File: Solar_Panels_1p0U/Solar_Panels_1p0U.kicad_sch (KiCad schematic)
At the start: 46 parts, among them J1 5040500891

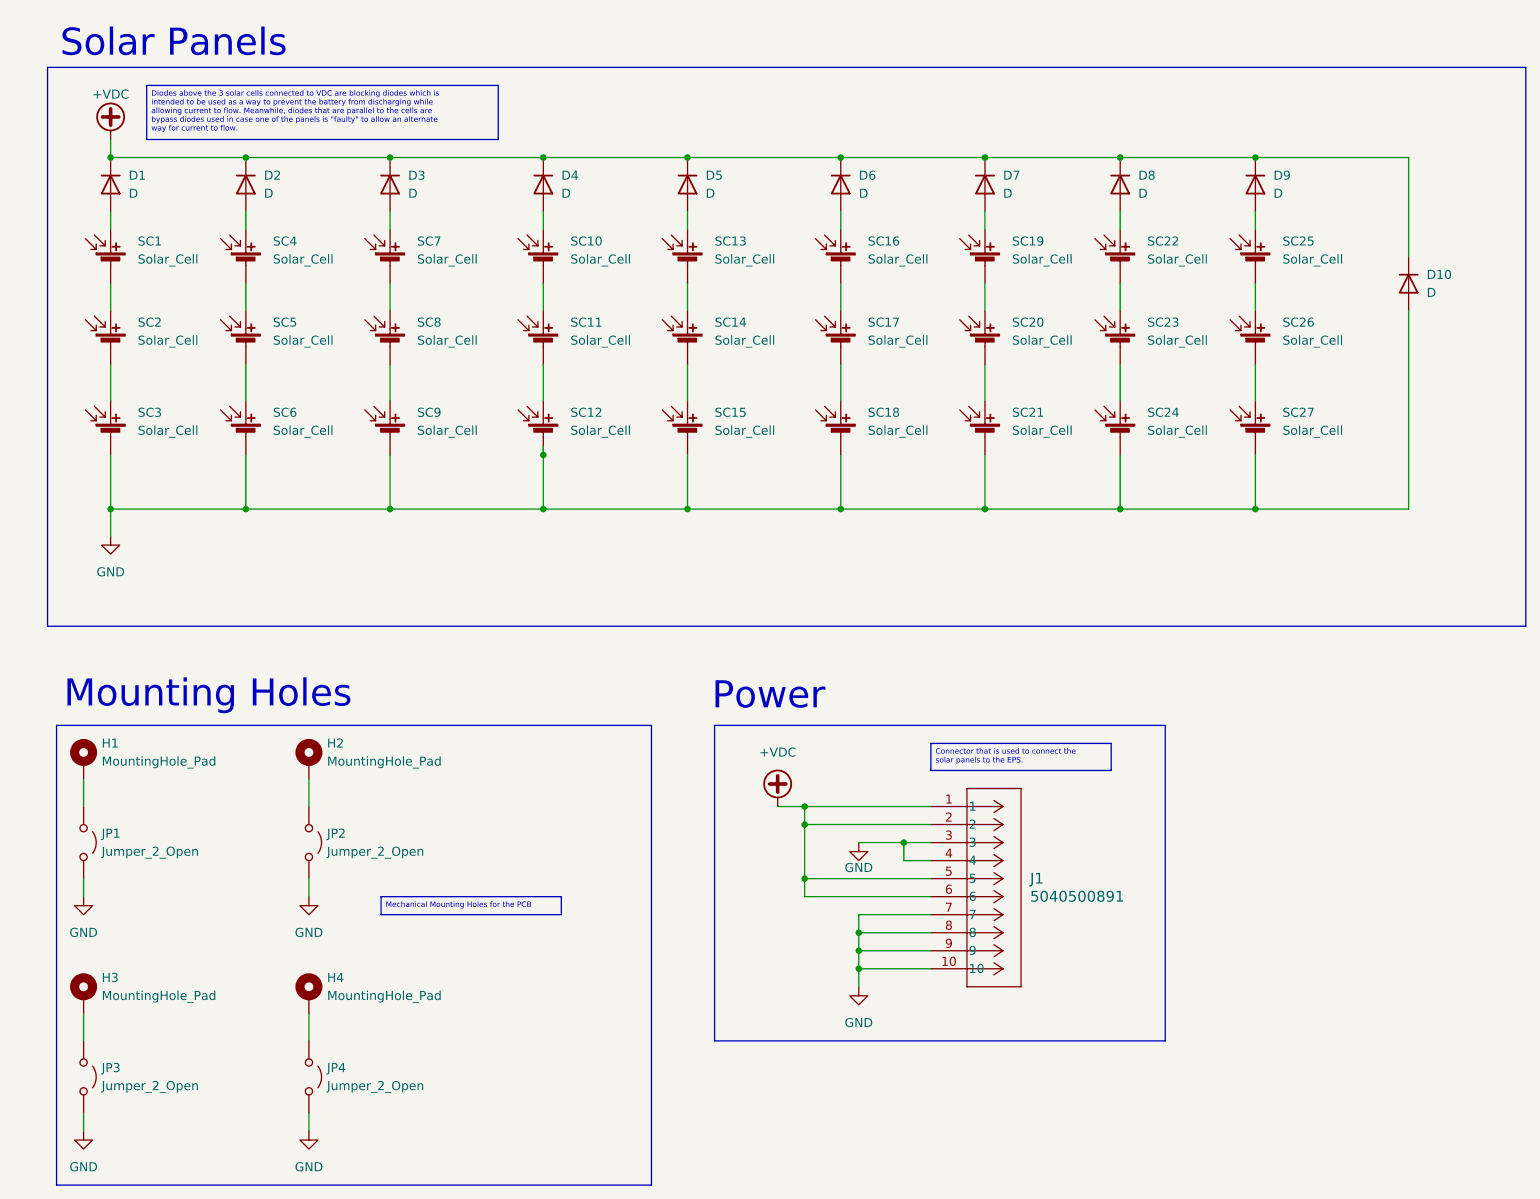
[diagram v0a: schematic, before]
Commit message: Kicad 9.0 PCB UPDATE
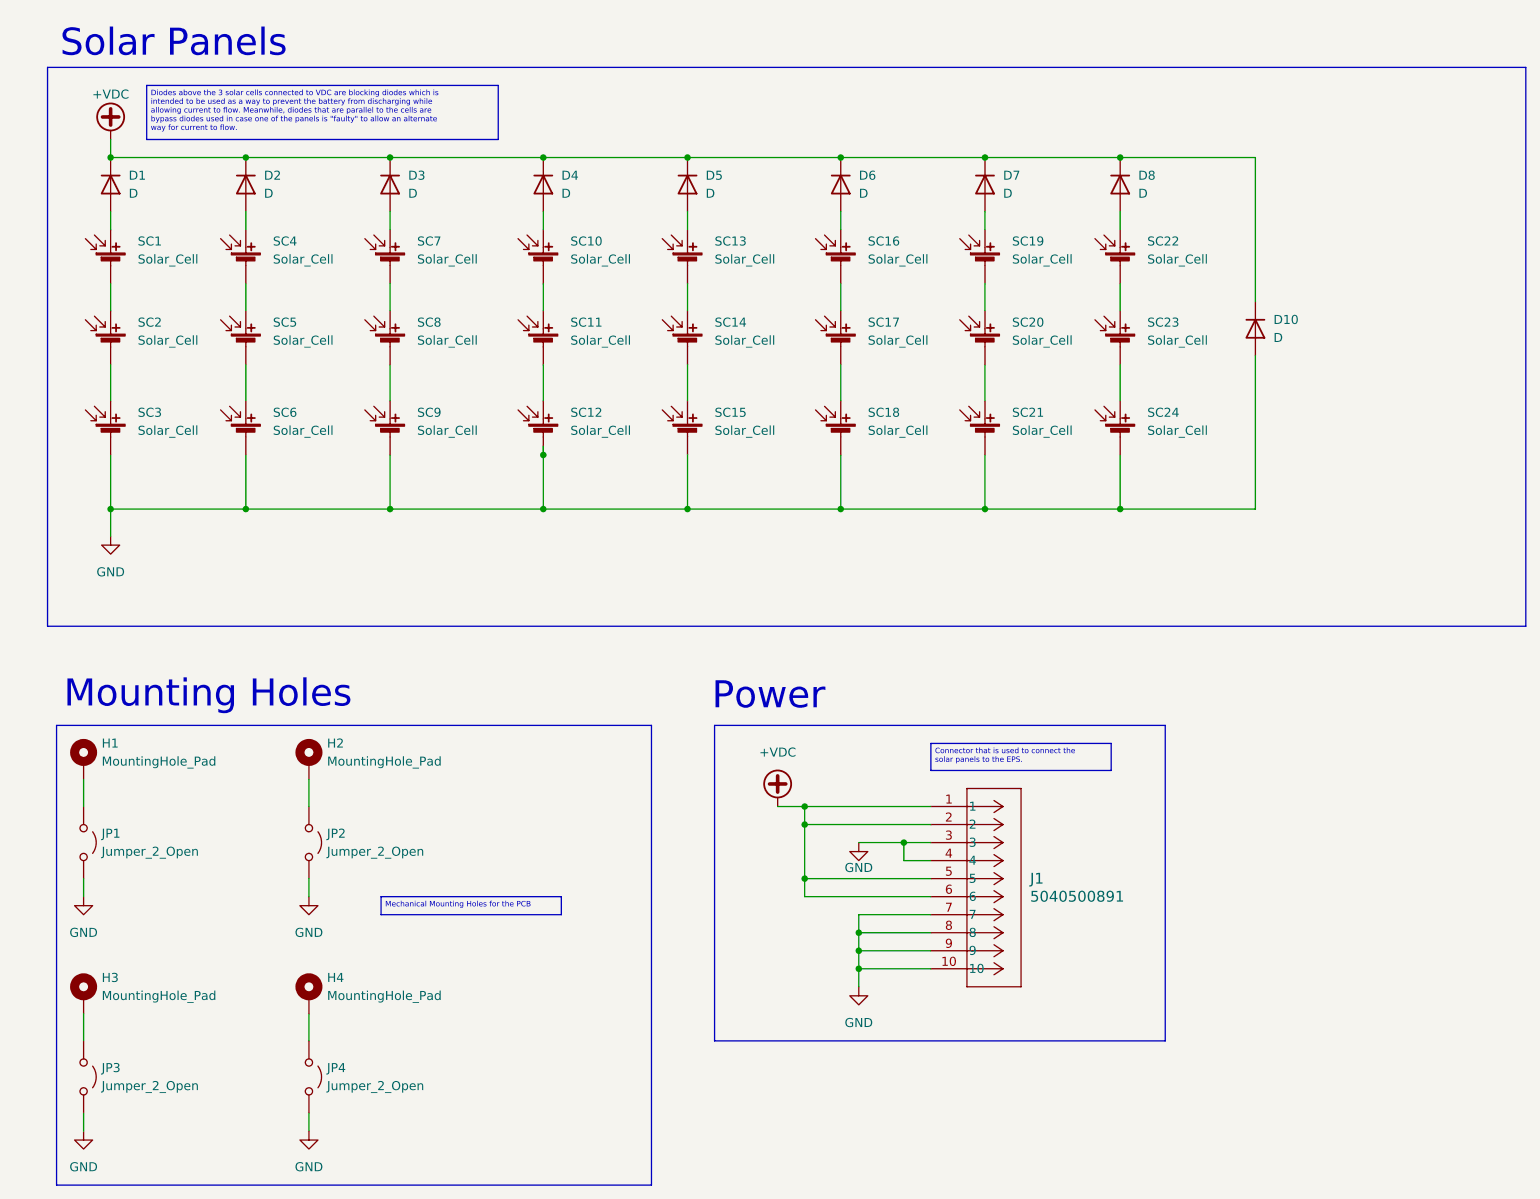
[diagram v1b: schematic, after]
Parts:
- removed D9: D, Solar Panels Library:PMEG10020AELPX, symbol Device:D
- removed SC25, SC26, SC27: Solar_Cell, Solar Panels Library:Trisolx Wings, symbol Device:Solar_Cell
- SC1, SC10, SC11, SC12, SC13, SC14, SC15, SC16, SC17, SC18, SC19, SC2, SC20, SC21, SC22, SC23, SC24, SC3, SC4, SC5, SC6, SC7, SC8, SC9: footprint Solar Panels Library:Trisolx Wings -> Solar Panels Library:TrisolX Solar Wings
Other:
- moved on the sheet: D10
